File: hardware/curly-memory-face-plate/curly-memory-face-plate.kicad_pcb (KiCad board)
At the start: 2 copper layers, 30 x 129 mm, 23 parts, among them J1 Thonkiconn_PJ398SM_panel, J2 Thonkiconn_PJ398SM_panel, J3 Thonkiconn_PJ398SM_panel, J4 Thonkiconn_PJ398SM_panel, J5 Thonkiconn_PJ398SM_panel, J6 Thonkiconn_PJ398SM_panel, J7 Thonkiconn_PJ398SM_panel, P1 2.54_pinheader_panel_01x05, P2 2.54_pinheader_panel_01x05, P3 2.54_pinheader_panel_01x05, P4 2.54_pinheader_panel_01x05, SW1 FSM14J_panel, SW2 FSM14J_panel, SW3 FSM14J_panel, SW4 FSM14J_panel

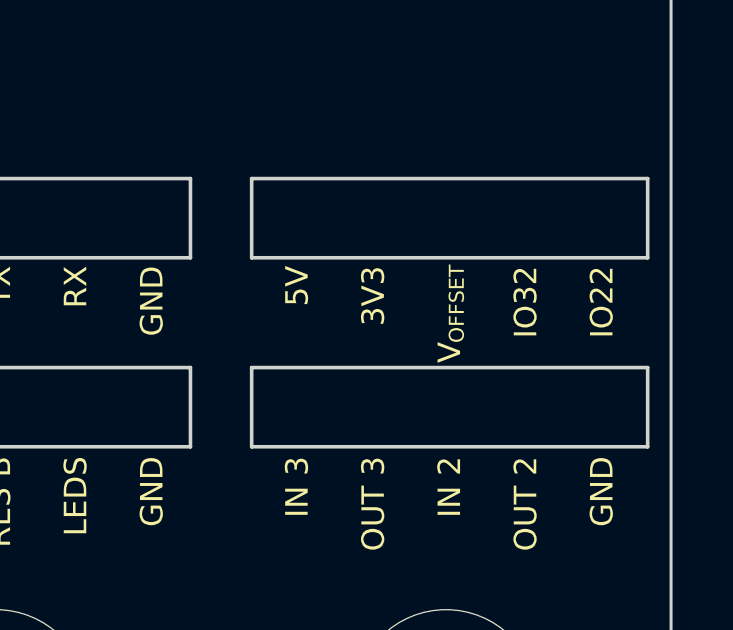
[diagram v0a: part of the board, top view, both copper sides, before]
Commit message: gerbers genearted and mf/mfpn added for main board for build
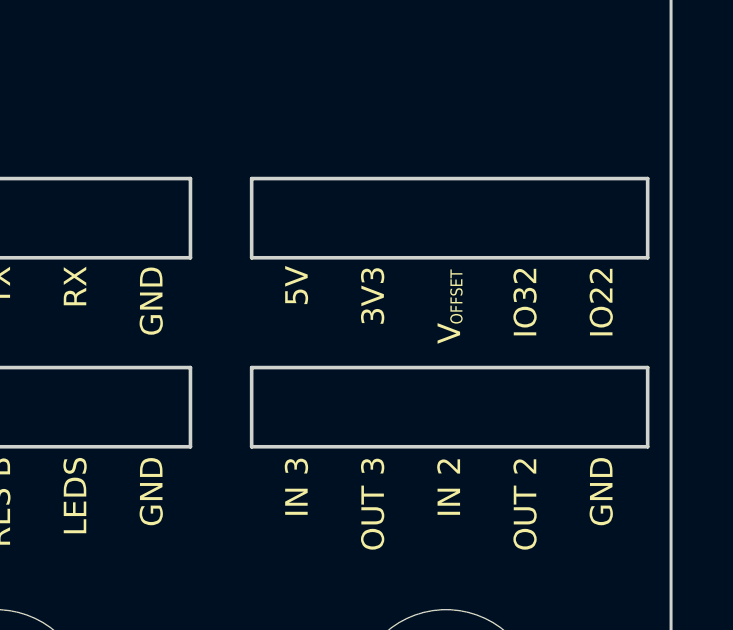
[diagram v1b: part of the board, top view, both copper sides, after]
